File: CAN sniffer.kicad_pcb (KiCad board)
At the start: 2 copper layers, 70.6 x 53.4 mm, 27 parts, among them J1 Conn_01x04, J2 Conn_01x04, U1 Nucleo_L432KC-MPPT-rescue, U2 ADM3055E-utsvt-chips, U3 CDSOT23-T24CAN-utsvt-chips

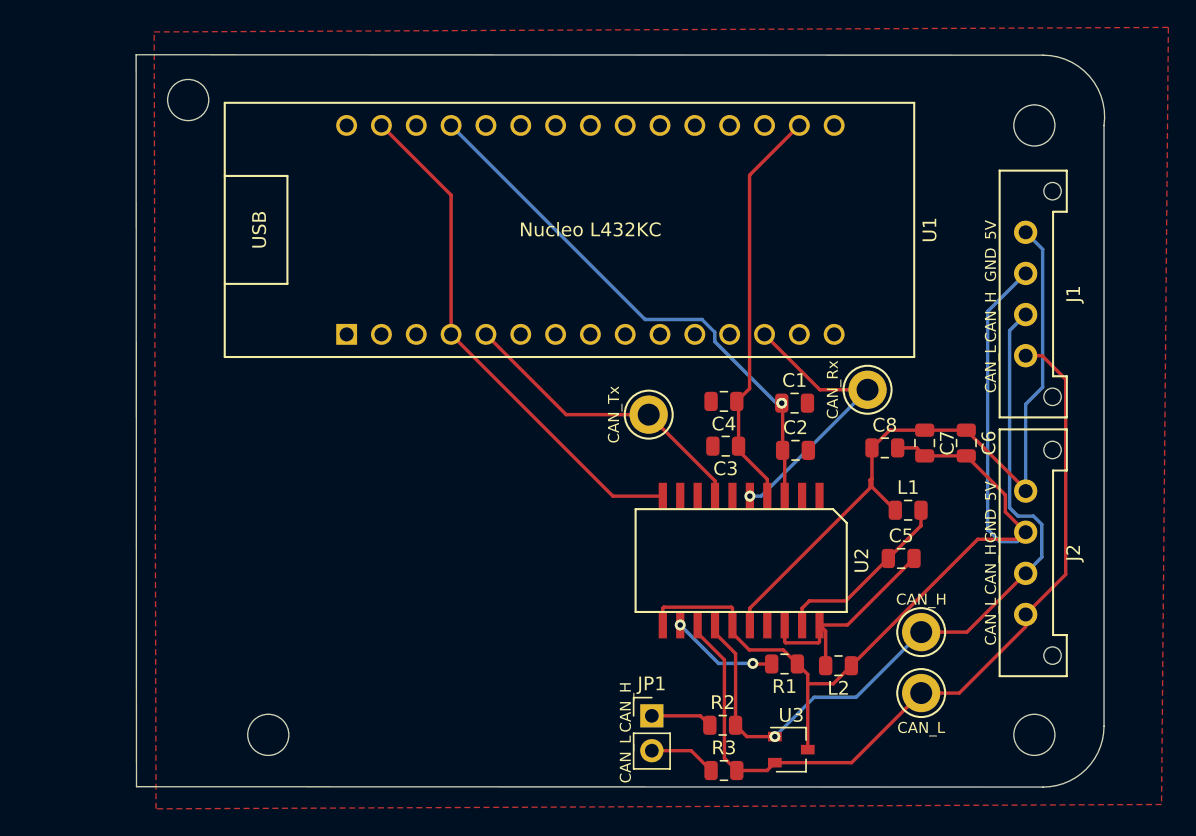
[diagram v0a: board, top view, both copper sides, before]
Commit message: Add files via upload
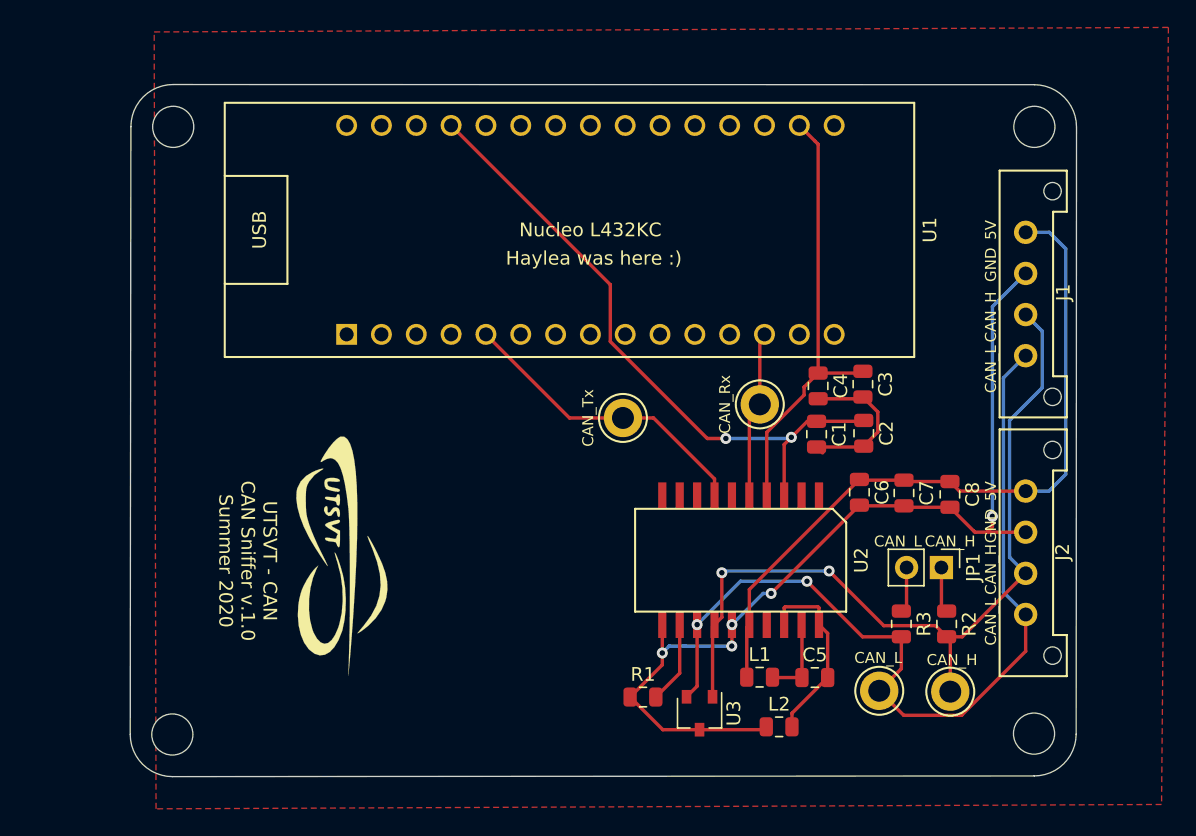
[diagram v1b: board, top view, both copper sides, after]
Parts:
- added G***: LOGO, UTSVT_Special:Hallock_Image_Small, B.Cu at (124.9, 97.3)
- added G***: LOGO, UTSVT_Special:UTSVT_Logo_Symbol, F.Cu at (115.1, 97.2)
- moved JP1 23.7 mm to (159.0, 98.3), turned to 270 degrees
- moved R2 17.9 mm to (159.3, 102.4), turned to 270 degrees
- moved R3 16.8 mm to (156.0, 102.4), turned to 270 degrees
- moved L1 16.3 mm to (145.7, 106.3)
- moved C3 11.0 mm to (153.2, 84.9), turned to 270 degrees
- moved C5 10.7 mm to (149.7, 106.3)
- moved R1 10.6 mm to (137.2, 107.7), turned to 0 degrees
- moved C6 8.59 mm to (153.0, 92.8)
- moved TP2 7.93 mm to (145.7, 86.4)
- moved U3 7.20 mm to (141.3, 108.9), turned to 270 degrees
- moved H3 7.00 mm to (102.9, 110.5)
- moved C4 6.96 mm to (150.0, 85.0), turned to 270 degrees
- moved L2 6.21 mm to (147.1, 109.9), turned to 0 degrees
- moved C8 5.84 mm to (159.6, 93.0), turned to 270 degrees
- moved C2 5.13 mm to (153.3, 88.5), turned to 270 degrees
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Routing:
- net GND: track 37.7 -> 11.9 mm
- net /CAN_Rx: track 21.0 -> 12.2 mm, vias 1 -> 0
- net Net-(C5-Pad1): track 13.5 -> 6.03 mm
- net +5V: track 39.8 -> 47.0 mm, vias 1 -> 2
- net Net-(C6-Pad2): track 76.8 -> 70.2 mm, vias 0 -> 5
- net /CAN_H: track 55.9 -> 60.4 mm, vias 1 -> 2
- net /CAN_L: track 60.1 -> 64.3 mm, vias 0 -> 2
- net Net-(C5-Pad2): track 17.1 -> 13.8 mm
- net +3V3: track 29.8 -> 32.4 mm
- net /RSlope: track 7.85 -> 6.00 mm, vias 2 -> 0
- net Net-(JP1-Pad2): track 4.92 -> 3.34 mm
- net Net-(JP1-Pad1): track 4.52 -> 3.34 mm
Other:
- board size 70.6 x 53.4 mm -> 69 x 50.5 mm
- board text added: "Dr. Gary Hallock"
- board text added: "Haylea was here :)"
- board text added: "UTSVT - CAN CAN Sniffer v.1.0 Summer 2020"

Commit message: Add files via upload
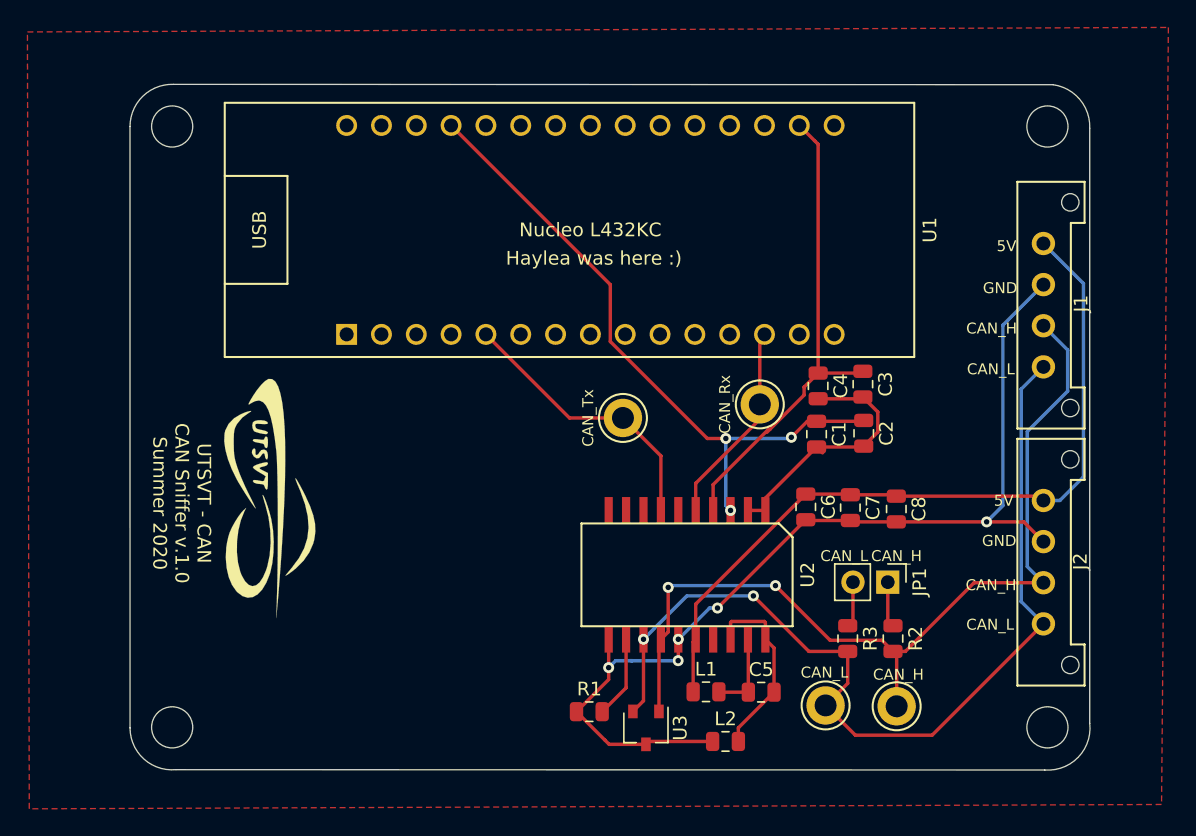
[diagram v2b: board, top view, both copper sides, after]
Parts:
- moved G*** 6.73 mm to (109.8, 93.0)
- moved G*** 4.77 mm to (120.4, 95.6)
- moved C5 4.05 mm to (145.8, 107.4)
- moved L2 4.05 mm to (143.2, 111.0)
- moved R2 4.05 mm to (155.4, 103.5)
- moved U3 4.05 mm to (137.4, 110.0)
- moved JP1 4.05 mm to (155.0, 99.4)
- moved C6 4.05 mm to (149.1, 93.9)
- moved C7 4.05 mm to (152.3, 93.9)
- moved C8 4.05 mm to (155.7, 94.0)
- moved L1 4.05 mm to (141.8, 107.4)
- moved R1 4.05 mm to (133.3, 108.8)
- moved R3 4.05 mm to (152.1, 103.5)
- moved TP3 4.05 mm to (155.7, 108.4)
- moved TP4 4.05 mm to (150.5, 108.3)
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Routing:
- net GND: track 11.9 -> 19.3 mm
- net /CAN_H: track 60.4 -> 66.1 mm
- net Net-(C6-Pad2): track 70.2 -> 74.5 mm
- net /CAN_L: track 64.3 -> 68.3 mm
- net /CAN_Rx: track 12.2 -> 16.0 mm
- net Net-(C6-Pad1): track 53.6 -> 57.2 mm
- net +3V3: track 32.4 -> 35.5 mm
- net /CAN_Tx: track 22.3 -> 20.4 mm
- net +5V: track 47.0 -> 47.9 mm, vias 2 -> 3
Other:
- board size 69 x 50.5 mm -> 70 x 50 mm
